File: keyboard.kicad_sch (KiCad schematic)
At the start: 295 parts

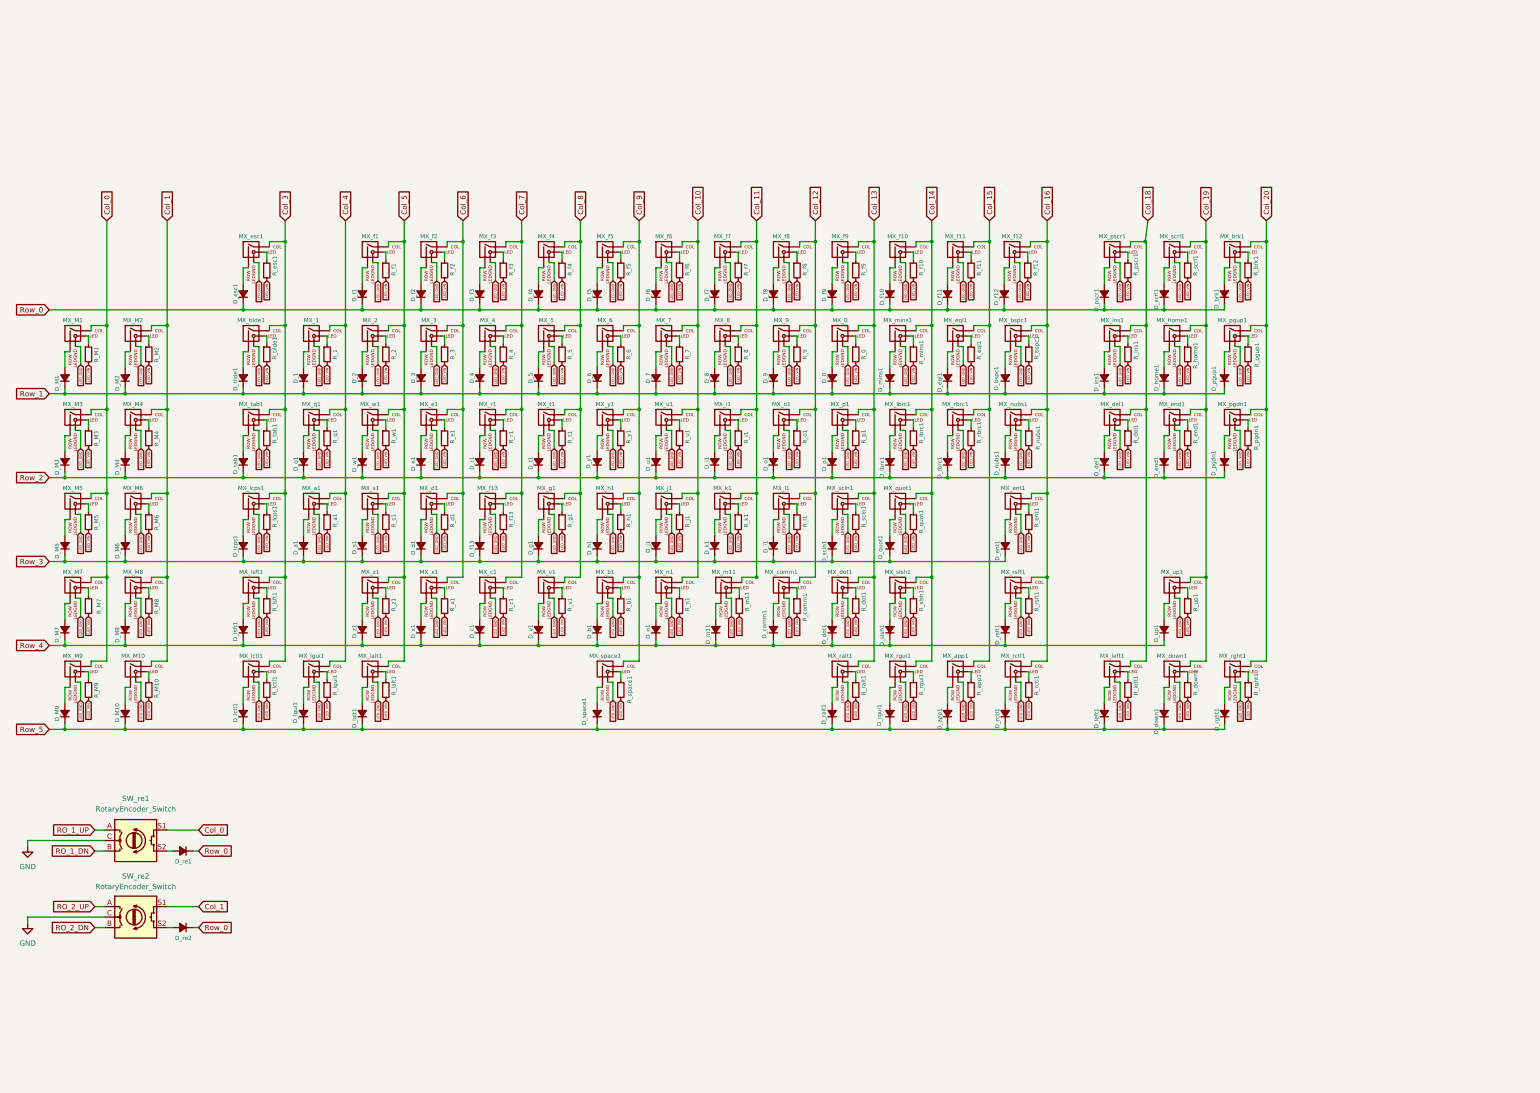
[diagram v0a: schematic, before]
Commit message: Update to plan
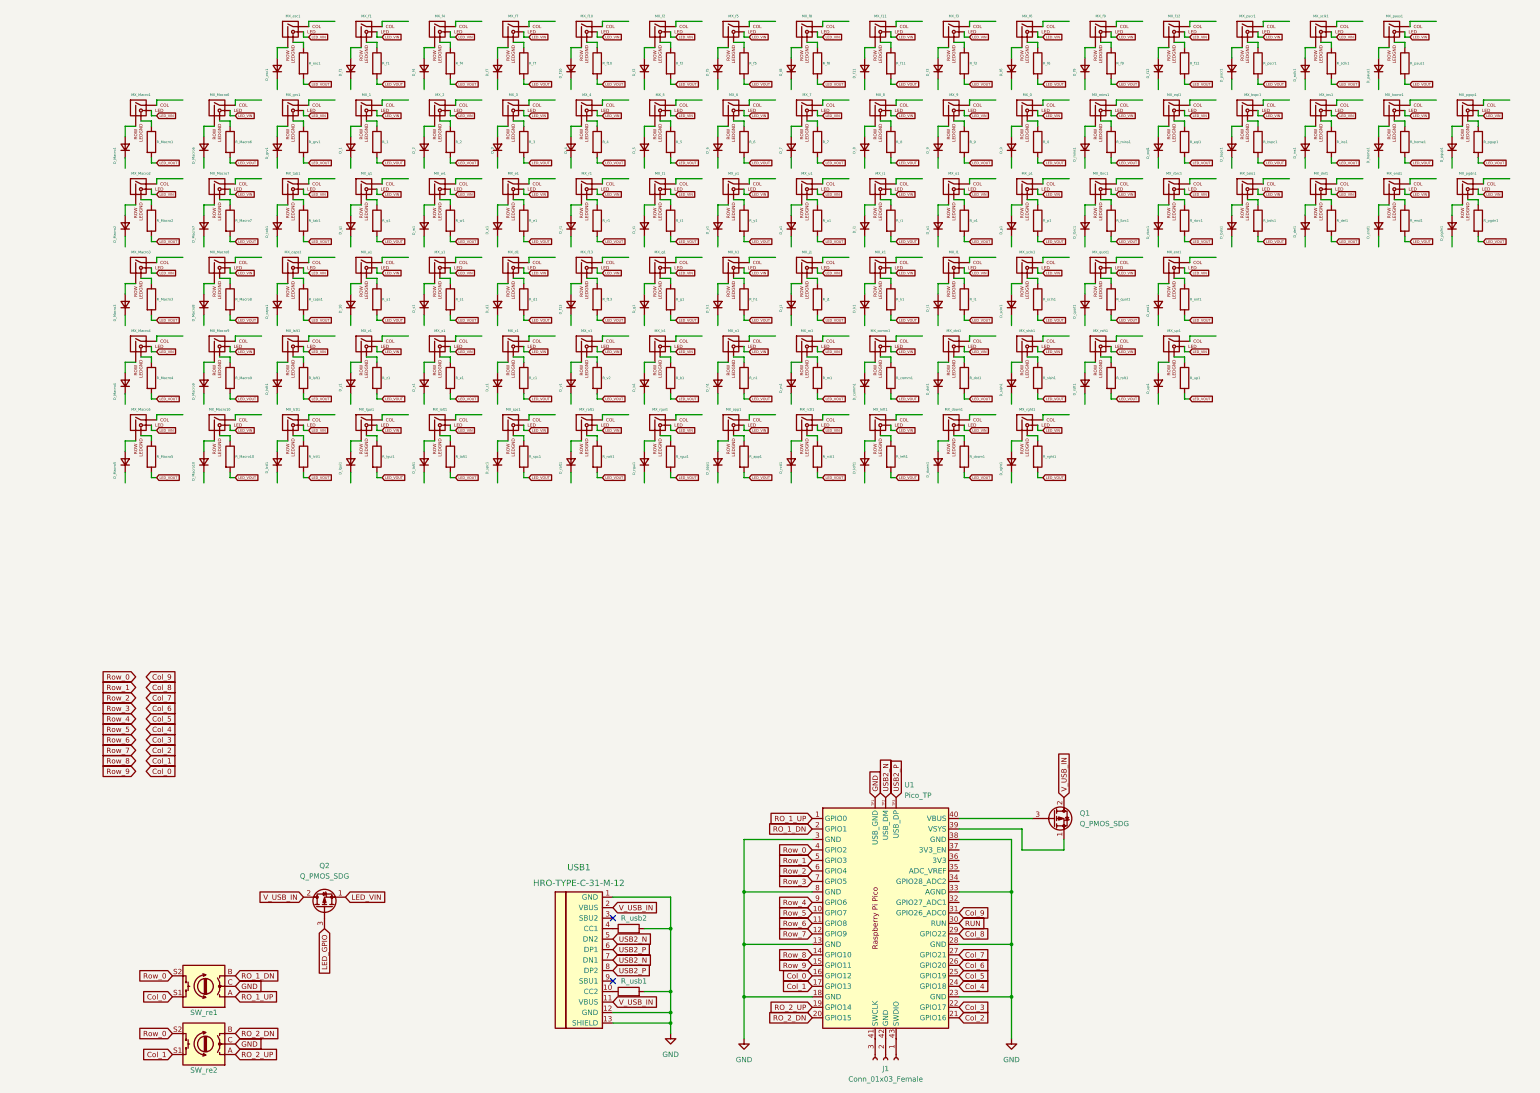
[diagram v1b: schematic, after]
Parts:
- removed D_0, D_1, D_2, D_3, D_4, D_5, D_6, D_7, D_8, D_9, D_M1, D_M10, D_M2, D_M3, D_M4, D_M5, D_M6, D_M7, D_M8, D_M9, D_a1, D_app1, D_b1, D_brk1, D_bspc1, D_c1, D_comm1, D_d1, D_del1, D_dot1, D_down1, D_e1, D_end1, D_ent1, D_eql1, D_esc1, D_f1, D_f10, D_f11, D_f12, D_f13, D_f2, D_f3, D_f4, D_f5, D_f6, D_f7, D_f8, D_f9, D_g1, D_h1, D_home1, D_i1, D_ins1, D_j1, D_k1, D_l1, D_lalt1, D_lbrc1, D_lcps1, D_lctl1, D_left1, D_lgui1, D_lsft1, D_m11, D_mins1, D_n1, D_nubs1, D_o1, D_p1, D_pgdn1, D_pgup1, D_pscr1, D_q1, D_quot1, D_r1, D_ralt1, D_rbrc1, D_rctl1, D_re1, D_re2, D_rght1, D_rgui1, D_rsft1, D_s1, D_scln1, D_scrl1, D_slsh1, D_space1, D_t1, D_tab1, D_tilde1, D_u1, D_up1, D_v1, D_w1, D_x1, D_y1, D_z1: D_Small_Filled, Diode_SMD:D_0805_2012Metric_Pad1.15x1.40mm_HandSolder, symbol Device:D_Small_Filled
- removed MX_M1, MX_M10, MX_M2, MX_M3, MX_M4, MX_M5, MX_M6, MX_M7, MX_M8, MX_M9, MX_brk1, MX_m11, MX_scrl1, MX_tilde1: MX-LED, 0_MX_Only:MXOnly-1U, symbol MX_Alps_Hybrid:MX-LED
- removed MX_lcps1: MX-LED, 0_MX_Only:MXOnly-1.75U, symbol MX_Alps_Hybrid:MX-LED
- removed MX_nubs1: MX-LED, 0_MX_Only:MXOnly-1.5U, symbol MX_Alps_Hybrid:MX-LED
- removed MX_space1: MX-LED, 0_MX_Only:MXOnly-6.25U-ReversedStabilizers, symbol MX_Alps_Hybrid:MX-LED
- removed R_0, R_1, R_2, R_3, R_4, R_5, R_6, R_7, R_8, R_9, R_M1, R_M10, R_M2, R_M3, R_M4, R_M5, R_M6, R_M7, R_M8, R_M9, R_a1, R_app1, R_b1, R_brk1, R_bspc1, R_c1, R_comm1, R_d1, R_del1, R_dot1, R_down1, R_e1, R_end1, R_ent1, R_eql1, R_esc1, R_f1, R_f10, R_f11, R_f12, R_f13, R_f2, R_f3, R_f4, R_f5, R_f6, R_f7, R_f8, R_f9, R_g1, R_h1, R_home1, R_i1, R_ins1, R_j1, R_k1, R_l1, R_lalt1, R_lbrc1, R_lcps1, R_lctl1, R_left1, R_lgui1, R_lsft1, R_m11, R_mins1, R_n1, R_nubs1, R_o1, R_p1, R_pgdn1, R_pgup1, R_pscr1, R_q1, R_quot1, R_r1, R_ralt1, R_rbrc1, R_rctl1, R_rght1, R_rgui1, R_rsft1, R_s1, R_scln1, R_scrl1, R_slsh1, R_space1, R_t1, R_tab1, R_tilde1, R_u1, R_up1, R_v1, R_w1, R_x1, R_y1, R_z1: R_Small, Resistor_SMD:R_0805_2012Metric_Pad1.20x1.40mm_HandSolder, symbol Device:R_Small
- added D_0, D_1, D_10, D_2, D_3, D_4, D_5, D_6, D_7, D_8, D_9, D_Macro1, D_Macro10, D_Macro2, D_Macro3, D_Macro4, D_Macro5, D_Macro6, D_Macro7, D_Macro8, D_Macro9, D_app1, D_b1, D_bsls1, D_bspc1, D_c1, D_caps1, D_comm1, D_d1, D_del1, D_dot1, D_down1, D_e1, D_end1, D_ent1, D_eql1, D_esc1, D_f1, D_f10, D_f11, D_f12, D_f13, D_f2, D_f3, D_f4, D_f5, D_f6, D_f7, D_f8, D_f9, D_g1, D_grv1, D_h1, D_home1, D_i1, D_ins1, D_j1, D_k1, D_l1, D_lalt1, D_lbrc1, D_lctl1, D_left1, D_lgui1, D_lsft1, D_m1, D_mins1, D_n1, D_o1, D_p1, D_paus1, D_pgdn1, D_pgup1, D_pscr1, D_q1, D_quot1, D_r1, D_ralt1, D_rbrc1, D_rctl1, D_rght1, D_rgui1, D_rsft1, D_s1, D_sclk1, D_scln1, D_slsh1, D_spc1, D_t1, D_tab1, D_u1, D_up1, D_v1, D_w1, D_x1, D_y1, D_z1: D_Small, symbol Device:D_Small
- added J1: Conn_01x03_Female, symbol Connector:Conn_01x03_Female
- added MX_Macro1, MX_Macro10, MX_Macro2, MX_Macro3, MX_Macro4, MX_Macro5, MX_Macro6, MX_Macro7, MX_Macro8, MX_Macro9, MX_grv1, MX_m1, MX_paus1, MX_sclk1: MX-LED, 0_MX_Only:MXOnly-1U, symbol MX_Alps_Hybrid:MX-LED
- added MX_bsls1: MX-LED, 0_MX_Only:MXOnly-1.5U, symbol MX_Alps_Hybrid:MX-LED
- added MX_caps1: MX-LED, 0_MX_Only:MXOnly-1.75U, symbol MX_Alps_Hybrid:MX-LED
- added MX_spc1: MX-LED, 0_MX_Only:MXOnly-6.25U-ReversedStabilizers, symbol MX_Alps_Hybrid:MX-LED
- added Q1, Q2: Q_PMOS_SDG, symbol Device:Q_PMOS_SDG
- added R_0, R_1, R_2, R_3, R_4, R_5, R_6, R_7, R_8, R_9, R_Macro1, R_Macro10, R_Macro2, R_Macro3, R_Macro4, R_Macro5, R_Macro6, R_Macro7, R_Macro8, R_Macro9, R_a1, R_app1, R_b1, R_bsls1, R_bspc1, R_c1, R_caps1, R_comm1, R_d1, R_del1, R_dot1, R_down1, R_e1, R_end1, R_ent1, R_eql1, R_esc1, R_f1, R_f10, R_f11, R_f12, R_f13, R_f2, R_f3, R_f4, R_f5, R_f6, R_f7, R_f8, R_f9, R_g1, R_grv1, R_h1, R_home1, R_i1, R_ins1, R_j1, R_k1, R_l1, R_lalt1, R_lbrc1, R_lctl1, R_left1, R_lgui1, R_lsft1, R_m1, R_mins1, R_n1, R_o1, R_p1, R_paus1, R_pgdn1, R_pgup1, R_pscr1, R_q1, R_quot1, R_r1, R_ralt1, R_rbrc1, R_rctl1, R_rght1, R_rgui1, R_rsft1, R_s1, R_sclk1, R_scln1, R_slsh1, R_spc1, R_t1, R_tab1, R_u1, R_up1, R_usb1, R_v2, R_w1, R_x1, R_y1, R_z1: R, symbol Device:R
- added R_usb2: 1, symbol Device:R
- added U1: Pico_TP, 0_MCU_RaspberryPi_and_Boards:RPi_Pico_SMD_TP, symbol 00_MCU_RaspberryPi_and_Boards:Pico_TP
- added USB1: HRO-TYPE-C-31-M-12, 0_Keebio:HRO-TYPE-C-31-M-12-Assembly, symbol 00_keebio:HRO-TYPE-C-31-M-12
- MX_bspc1: footprint 0_MX_Only:MXOnly-2U-ReversedStabilizers -> 0_MX_Only:MXOnly-2U
- MX_rgui1: footprint 0_MX_Only:MXOnly-1U -> 0_MX_Only:MXOnly-1.25U
- SW_re1, SW_re2: footprint keebio:RotaryEncoder_Alps_EC11E-Switch_Vertical_H20mm -> 0_Keebio:RotaryEncoder_EC11
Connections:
- net Col_0: now also U1.16 (GPIO12)
- net Col_1: now also U1.17 (GPIO13)
- net Col_3: now also U1.22 (GPIO17); no longer MX_esc1.1 (COL), MX_lctl1.1 (COL), MX_lsft1.1 (COL), MX_tab1.1 (COL)
- net Col_4: now also U1.24 (GPIO18); no longer MX_1.1 (COL), MX_a1.1 (COL), MX_lgui1.1 (COL), MX_q1.1 (COL)
- net Col_5: now also U1.25 (GPIO19); no longer MX_2.1 (COL), MX_f1.1 (COL), MX_lalt1.1 (COL), MX_s1.1 (COL), MX_w1.1 (COL), MX_z1.1 (COL)
- net Col_6: now also U1.26 (GPIO20); no longer MX_3.1 (COL), MX_d1.1 (COL), MX_e1.1 (COL), MX_f2.1 (COL), MX_x1.1 (COL)
- net Col_7: now also U1.27 (GPIO21); no longer MX_4.1 (COL), MX_c1.1 (COL), MX_f13.1 (COL), MX_f3.1 (COL), MX_r1.1 (COL)
- net Col_8: now also U1.29 (GPIO22); no longer MX_5.1 (COL), MX_f4.1 (COL), MX_g1.1 (COL), MX_t1.1 (COL), MX_v1.1 (COL)
- net Col_9: now also U1.31 (GPIO26_ADC0); no longer MX_6.1 (COL), MX_b1.1 (COL), MX_f5.1 (COL), MX_h1.1 (COL), MX_y1.1 (COL)
- net GND: now also R_usb1.2, R_usb2.2, U1.13 (GND), U1.18 (GND), U1.23 (GND), U1.28 (GND), U1.3 (GND), U1.33 (AGND), U1.38 (GND), U1.8 (GND), U1.TP1 (USB_GND), USB1.1 (GND), USB1.12 (GND), USB1.13 (SHIELD)
- net LED_VIN: now also MX_0.3 (LED), MX_1.3 (LED), MX_2.3 (LED), MX_3.3 (LED), MX_4.3 (LED), MX_5.3 (LED), MX_6.3 (LED), MX_7.3 (LED), MX_8.3 (LED), MX_9.3 (LED), MX_a1.3 (LED), MX_app1.3 (LED), MX_b1.3 (LED), MX_bspc1.3 (LED), MX_c1.3 (LED), MX_comm1.3 (LED), MX_d1.3 (LED), MX_del1.3 (LED), MX_dot1.3 (LED), MX_down1.3 (LED), MX_e1.3 (LED), MX_end1.3 (LED), MX_ent1.3 (LED), MX_eql1.3 (LED), MX_esc1.3 (LED), MX_f1.3 (LED), MX_f10.3 (LED), MX_f11.3 (LED), MX_f12.3 (LED), MX_f13.3 (LED), MX_f2.3 (LED), MX_f3.3 (LED), MX_f4.3 (LED), MX_f5.3 (LED), MX_f6.3 (LED), MX_f7.3 (LED), MX_f8.3 (LED), MX_f9.3 (LED), MX_g1.3 (LED), MX_h1.3 (LED), MX_home1.3 (LED), MX_i1.3 (LED), MX_ins1.3 (LED), MX_j1.3 (LED), MX_k1.3 (LED), MX_l1.3 (LED), MX_lalt1.3 (LED), MX_lbrc1.3 (LED), MX_lctl1.3 (LED), MX_left1.3 (LED), MX_lgui1.3 (LED), MX_lsft1.3 (LED), MX_mins1.3 (LED), MX_n1.3 (LED), MX_o1.3 (LED), MX_p1.3 (LED), MX_pgdn1.3 (LED), MX_pgup1.3 (LED), MX_pscr1.3 (LED), MX_q1.3 (LED), MX_quot1.3 (LED), MX_r1.3 (LED), MX_ralt1.3 (LED), MX_rbrc1.3 (LED), MX_rctl1.3 (LED), MX_rght1.3 (LED), MX_rgui1.3 (LED), MX_rsft1.3 (LED), MX_s1.3 (LED), MX_scln1.3 (LED), MX_slsh1.3 (LED), MX_t1.3 (LED), MX_tab1.3 (LED), MX_u1.3 (LED), MX_up1.3 (LED), MX_v1.3 (LED), MX_w1.3 (LED), MX_x1.3 (LED), MX_y1.3 (LED), MX_z1.3 (LED), MX_Macro1.3 (LED), MX_Macro10.3 (LED), MX_Macro2.3 (LED), MX_Macro3.3 (LED), MX_Macro4.3 (LED), MX_Macro5.3 (LED), MX_Macro6.3 (LED), MX_Macro7.3 (LED), MX_Macro8.3 (LED), MX_Macro9.3 (LED), MX_bsls1.3 (LED), MX_caps1.3 (LED), MX_grv1.3 (LED), MX_m1.3 (LED), MX_paus1.3 (LED), MX_sclk1.3 (LED), MX_spc1.3 (LED), Q2.1 (S)
- net RO_1_UP: now also U1.1 (GPIO0)
- net RO_2_DN: now also U1.20 (GPIO15)
- net RO_2_UP: now also U1.19 (GPIO14)
- net Row_0: now also SW_re1.S2, SW_re2.S2, U1.4 (GPIO2)
- net Row_1: now also U1.5 (GPIO3)
- net Row_2: now also U1.6 (GPIO4)
- net Row_3: now also U1.7 (GPIO5)
- net Row_4: now also U1.9 (GPIO6)
- net Row_5: now also U1.10 (GPIO7)
- net at MX_pscr1.2 (ROW): now also D_pscr1.2 (A)
- net at MX_p1.2 (ROW): now also D_p1.2 (A)
- net at MX_end1.2 (ROW): now also D_end1.2 (A)
- net at MX_ralt1.2 (ROW): now also D_ralt1.2 (A)
- net at MX_o1.2 (ROW): now also D_o1.2 (A)
- net at MX_4.2 (ROW): now also D_4.2 (A)
- net at MX_y1.2 (ROW): now also D_y1.2 (A)
- net at MX_l1.2 (ROW): now also D_l1.2 (A)
- net at MX_6.2 (ROW): now also D_6.2 (A)
- net at MX_pgup1.2 (ROW): now also D_pgup1.2 (A)
- net at MX_eql1.2 (ROW): now also D_eql1.2 (A)
- net at MX_n1.2 (ROW): now also D_n1.2 (A)
- net at MX_j1.2 (ROW): now also D_j1.2 (A)
- net at MX_f5.2 (ROW): now also D_f5.2 (A)
- net at MX_f3.2 (ROW): now also D_f3.2 (A)
- net at MX_f7.2 (ROW): now also D_f7.2 (A)
- net at MX_rght1.2 (ROW): now also D_rght1.2 (A)
- net at MX_u1.2 (ROW): now also D_u1.2 (A)
- net at MX_rbrc1.2 (ROW): now also D_rbrc1.2 (A)
- net at MX_7.2 (ROW): now also D_7.2 (A)
- net at MX_pgdn1.2 (ROW): now also D_pgdn1.2 (A)
- net at MX_mins1.2 (ROW): now also D_mins1.2 (A)
- net at MX_x1.2 (ROW): now also D_x1.2 (A)
- net at MX_f4.2 (ROW): now also D_f4.2 (A)
- net at MX_f9.2 (ROW): now also D_f9.2 (A)
- net at MX_b1.2 (ROW): now also D_b1.2 (A)
- net at MX_dot1.2 (ROW): now also D_dot1.2 (A)
- net at MX_left1.2 (ROW): now also D_left1.2 (A)
- net at MX_f12.2 (ROW): now also D_f12.2 (A)
- net at MX_lalt1.2 (ROW): now also D_lalt1.2 (A)
- net at MX_r1.2 (ROW): now also D_r1.2 (A)
- net at MX_3.2 (ROW): now also D_3.2 (A)
- net at MX_g1.2 (ROW): now also D_g1.2 (A)
- net at MX_ent1.2 (ROW): now also D_ent1.2 (A)
- net at MX_1.2 (ROW): now also D_1.2 (A)
- net at MX_k1.2 (ROW): now also D_k1.2 (A)
- net at MX_f8.2 (ROW): now also D_f8.2 (A)
- net at MX_ins1.2 (ROW): now also D_ins1.2 (A)
- net at MX_c1.2 (ROW): now also D_c1.2 (A)
- net at MX_rsft1.2 (ROW): now also D_rsft1.2 (A)
- net at MX_f10.2 (ROW): now also D_f10.2 (A)
- net at MX_z1.2 (ROW): now also D_z1.2 (A)
- net at MX_e1.2 (ROW): now also D_e1.2 (A)
- net at MX_f1.2 (ROW): now also D_f1.2 (A)
- net at MX_d1.2 (ROW): now also D_d1.2 (A)
- net at MX_t1.2 (ROW): now also D_t1.2 (A)
- net at MX_9.2 (ROW): now also D_9.2 (A)
- net at MX_w1.2 (ROW): now also D_w1.2 (A)
- net at MX_0.2 (ROW): now also D_0.2 (A)
- net at MX_rgui1.2 (ROW): now also D_rgui1.2 (A)
- net at MX_home1.2 (ROW): now also D_home1.2 (A)
- net at MX_bspc1.2 (ROW): now also D_bspc1.2 (A)
- net at MX_s1.2 (ROW): now also D_s1.2 (A)
- net at MX_rctl1.2 (ROW): now also D_rctl1.2 (A)
- net at MX_8.2 (ROW): now also D_8.2 (A)
- net at MX_quot1.2 (ROW): now also D_quot1.2 (A)
- net at MX_comm1.2 (ROW): now also D_comm1.2 (A)
- net at MX_f11.2 (ROW): now also D_f11.2 (A)
- net at MX_del1.2 (ROW): now also D_del1.2 (A)
- net at MX_lgui1.2 (ROW): now also D_lgui1.2 (A)
- net at MX_v1.2 (ROW): now also D_v1.2 (A)
- net at MX_h1.2 (ROW): now also D_h1.2 (A)
- net at MX_slsh1.2 (ROW): now also D_slsh1.2 (A)
- net at MX_lsft1.2 (ROW): now also D_lsft1.2 (A)
- net at MX_lbrc1.2 (ROW): now also D_lbrc1.2 (A)
- net at MX_tab1.2 (ROW): now also D_tab1.2 (A)
- net at MX_f13.2 (ROW): now also D_f13.2 (A)
- net at MX_f6.2 (ROW): now also D_f6.2 (A)
- net at MX_5.2 (ROW): now also D_5.2 (A)
- net at MX_scln1.2 (ROW): now also D_scln1.2 (A)
- net at MX_app1.2 (ROW): now also D_app1.2 (A)
- net at MX_a1.2 (ROW): now also D_10.2 (A)
- net at MX_down1.2 (ROW): now also D_down1.2 (A)
- net at MX_q1.2 (ROW): now also D_q1.2 (A)
- net at MX_f2.2 (ROW): now also D_f2.2 (A)
- net at MX_esc1.2 (ROW): now also D_esc1.2 (A)
- net at MX_lctl1.2 (ROW): now also D_lctl1.2 (A)
- net at MX_i1.2 (ROW): now also D_i1.2 (A)
- net at MX_up1.2 (ROW): now also D_up1.2 (A)
- net at MX_2.2 (ROW): now also D_2.2 (A)
- removed net Col_10: MX_7.1 (COL), MX_f6.1 (COL), MX_j1.1 (COL), MX_n1.1 (COL), MX_u1.1 (COL)
- removed net Col_11: MX_8.1 (COL), MX_f7.1 (COL), MX_i1.1 (COL), MX_k1.1 (COL)
- removed net Col_12: MX_9.1 (COL), MX_comm1.1 (COL), MX_f8.1 (COL), MX_l1.1 (COL), MX_o1.1 (COL)
- removed net Col_13: MX_0.1 (COL), MX_dot1.1 (COL), MX_f9.1 (COL), MX_p1.1 (COL), MX_ralt1.1 (COL), MX_scln1.1 (COL)
- removed net Col_14: MX_f10.1 (COL), MX_lbrc1.1 (COL), MX_mins1.1 (COL), MX_quot1.1 (COL), MX_rgui1.1 (COL), MX_slsh1.1 (COL)
- removed net Col_15: MX_app1.1 (COL), MX_eql1.1 (COL), MX_f11.1 (COL), MX_rbrc1.1 (COL)
- removed net Col_16: MX_bspc1.1 (COL), MX_ent1.1 (COL), MX_f12.1 (COL), MX_rctl1.1 (COL), MX_rsft1.1 (COL)
- removed net Col_18: MX_del1.1 (COL), MX_ins1.1 (COL), MX_left1.1 (COL), MX_pscr1.1 (COL)
- removed net Col_19: MX_down1.1 (COL), MX_end1.1 (COL), MX_home1.1 (COL), MX_up1.1 (COL)
- removed net Col_20: MX_pgdn1.1 (COL), MX_pgup1.1 (COL), MX_rght1.1 (COL)
- removed net LED_GND: MX_0.4 (LEDGND), MX_1.4 (LEDGND), MX_2.4 (LEDGND), MX_3.4 (LEDGND), MX_4.4 (LEDGND), MX_5.4 (LEDGND), MX_6.4 (LEDGND), MX_7.4 (LEDGND), MX_8.4 (LEDGND), MX_9.4 (LEDGND), MX_a1.4 (LEDGND), MX_app1.4 (LEDGND), MX_b1.4 (LEDGND), MX_bspc1.4 (LEDGND), MX_c1.4 (LEDGND), MX_comm1.4 (LEDGND), MX_d1.4 (LEDGND), MX_del1.4 (LEDGND), MX_dot1.4 (LEDGND), MX_down1.4 (LEDGND), MX_e1.4 (LEDGND), MX_end1.4 (LEDGND), MX_ent1.4 (LEDGND), MX_eql1.4 (LEDGND), MX_esc1.4 (LEDGND), MX_f1.4 (LEDGND), MX_f10.4 (LEDGND), MX_f11.4 (LEDGND), MX_f12.4 (LEDGND), MX_f13.4 (LEDGND), MX_f2.4 (LEDGND), MX_f3.4 (LEDGND), MX_f4.4 (LEDGND), MX_f5.4 (LEDGND), MX_f6.4 (LEDGND), MX_f7.4 (LEDGND), MX_f8.4 (LEDGND), MX_f9.4 (LEDGND), MX_g1.4 (LEDGND), MX_h1.4 (LEDGND), MX_home1.4 (LEDGND), MX_i1.4 (LEDGND), MX_ins1.4 (LEDGND), MX_j1.4 (LEDGND), MX_k1.4 (LEDGND), MX_l1.4 (LEDGND), MX_lalt1.4 (LEDGND), MX_lbrc1.4 (LEDGND), MX_lctl1.4 (LEDGND), MX_left1.4 (LEDGND), MX_lgui1.4 (LEDGND), MX_lsft1.4 (LEDGND), MX_mins1.4 (LEDGND), MX_n1.4 (LEDGND), MX_o1.4 (LEDGND), MX_p1.4 (LEDGND), MX_pgdn1.4 (LEDGND), MX_pgup1.4 (LEDGND), MX_pscr1.4 (LEDGND), MX_q1.4 (LEDGND), MX_quot1.4 (LEDGND), MX_r1.4 (LEDGND), MX_ralt1.4 (LEDGND), MX_rbrc1.4 (LEDGND), MX_rctl1.4 (LEDGND), MX_rght1.4 (LEDGND), MX_rgui1.4 (LEDGND), MX_rsft1.4 (LEDGND), MX_s1.4 (LEDGND), MX_scln1.4 (LEDGND), MX_slsh1.4 (LEDGND), MX_t1.4 (LEDGND), MX_tab1.4 (LEDGND), MX_u1.4 (LEDGND), MX_up1.4 (LEDGND), MX_v1.4 (LEDGND), MX_w1.4 (LEDGND), MX_x1.4 (LEDGND), MX_y1.4 (LEDGND), MX_z1.4 (LEDGND)
- new net: MX_f7.4 (LEDGND), R_f7.1
- new net: D_m1.2 (A), MX_m1.2 (ROW)
- new net: MX_ralt1.4 (LEDGND), R_ralt1.1
- new net: MX_pscr1.4 (LEDGND), R_pscr1.1
- new net: J1.1 (Pin_1), U1.43 (SWDIO)
- new net: J1.2 (Pin_2), U1.42 (GND)
- new net: J1.3 (Pin_3), U1.41 (SWCLK)
- new net: MX_pgdn1.4 (LEDGND), R_pgdn1.1
- new net: MX_p1.4 (LEDGND), R_p1.1
- new net: MX_f1.4 (LEDGND), R_f1.1
- new net: MX_3.4 (LEDGND), R_3.1
- new net: D_caps1.2 (A), MX_caps1.2 (ROW)
- new net: MX_caps1.4 (LEDGND), R_caps1.1
- new net: MX_y1.4 (LEDGND), R_y1.1
- new net: MX_r1.4 (LEDGND), R_r1.1
- new net: MX_ins1.4 (LEDGND), R_ins1.1
- new net: MX_Macro1.4 (LEDGND), R_Macro1.1
- new net: MX_f2.4 (LEDGND), R_f2.1
- new net: MX_f10.4 (LEDGND), R_f10.1
- new net: MX_quot1.4 (LEDGND), R_quot1.1
- new net: MX_esc1.4 (LEDGND), R_esc1.1
- new net: MX_q1.4 (LEDGND), R_q1.1
- new net: MX_lalt1.4 (LEDGND), R_lalt1.1
- new net: D_bsls1.2 (A), MX_bsls1.2 (ROW)
- new net: MX_bsls1.4 (LEDGND), R_bsls1.1
- new net: MX_dot1.4 (LEDGND), R_dot1.1
- new net: MX_5.4 (LEDGND), R_5.1
- new net: MX_down1.4 (LEDGND), R_down1.1
- new net: MX_tab1.4 (LEDGND), R_tab1.1
- new net: R_usb1.1, USB1.10 (CC2)
- new net: R_usb2.1, USB1.4 (CC1)
- new net: MX_scln1.4 (LEDGND), R_scln1.1
- new net: MX_f13.4 (LEDGND), R_f13.1
- new net: MX_d1.4 (LEDGND), R_d1.1
- new net: MX_x1.4 (LEDGND), R_x1.1
- new net: D_Macro9.2 (A), MX_Macro9.2 (ROW)
- new net: MX_rgui1.4 (LEDGND), R_rgui1.1
- new net: MX_e1.4 (LEDGND), R_e1.1
- new net: MX_f5.4 (LEDGND), R_f5.1
- new net: D_spc1.2 (A), MX_spc1.2 (ROW)
- new net: MX_spc1.4 (LEDGND), R_spc1.1
- new net: D_Macro1.2 (A), MX_Macro1.2 (ROW)
- new net: MX_f6.4 (LEDGND), R_f6.1
- new net: MX_b1.4 (LEDGND), R_b1.1
- new net: D_Macro8.2 (A), MX_Macro8.2 (ROW)
- new net: MX_Macro8.4 (LEDGND), R_Macro8.1
- new net: MX_l1.4 (LEDGND), R_l1.1
- new net: MX_t1.4 (LEDGND), R_t1.1
- new net: MX_Macro10.4 (LEDGND), R_Macro10.1
- new net: MX_eql1.4 (LEDGND), R_eql1.1
- new net: MX_rbrc1.4 (LEDGND), R_rbrc1.1
- new net: MX_v1.4 (LEDGND), R_v2.1
- new net: MX_lbrc1.4 (LEDGND), R_lbrc1.1
- new net: MX_4.4 (LEDGND), R_4.1
- new net: MX_8.4 (LEDGND), R_8.1
- new net: MX_a1.4 (LEDGND), R_a1.1
- new net: MX_f9.4 (LEDGND), R_f9.1
- new net: MX_rsft1.4 (LEDGND), R_rsft1.1
- new net: MX_home1.4 (LEDGND), R_home1.1
- new net: MX_h1.4 (LEDGND), R_h1.1
- new net: MX_f4.4 (LEDGND), R_f4.1
- new net: MX_k1.4 (LEDGND), R_k1.1
- new net: MX_rctl1.4 (LEDGND), R_rctl1.1
- new net: MX_1.4 (LEDGND), R_1.1
- new net: MX_up1.4 (LEDGND), R_up1.1
- new net: MX_m1.4 (LEDGND), R_m1.1
- new net: D_Macro6.2 (A), MX_Macro6.2 (ROW)
- new net: MX_comm1.4 (LEDGND), R_comm1.1
- new net: Q1.1 (S), U1.39 (VSYS)
- new net: Q1.3 (G), U1.40 (VBUS)
- new net: MX_s1.4 (LEDGND), R_s1.1
- new net: MX_7.4 (LEDGND), R_7.1
- new net: MX_o1.4 (LEDGND), R_o1.1
- new net: MX_Macro9.4 (LEDGND), R_Macro9.1
- new net: MX_del1.4 (LEDGND), R_del1.1
- new net: MX_pgup1.4 (LEDGND), R_pgup1.1
- new net: MX_z1.4 (LEDGND), R_z1.1
- new net: MX_left1.4 (LEDGND), R_left1.1
- new net: MX_slsh1.4 (LEDGND), R_slsh1.1
- new net: MX_u1.4 (LEDGND), R_u1.1
- new net: D_sclk1.2 (A), MX_sclk1.2 (ROW)
- new net: MX_rght1.4 (LEDGND), R_rght1.1
- new net: MX_2.4 (LEDGND), R_2.1
- new net: MX_mins1.4 (LEDGND), R_mins1.1
- new net: D_paus1.2 (A), MX_paus1.2 (ROW)
- new net: MX_g1.4 (LEDGND), R_g1.1
- new net: D_grv1.2 (A), MX_grv1.2 (ROW)
- new net: D_Macro10.2 (A), MX_Macro10.2 (ROW)
- new net: MX_grv1.4 (LEDGND), R_grv1.1
- new net: MX_Macro5.4 (LEDGND), R_Macro5.1
- new net: MX_6.4 (LEDGND), R_6.1
- new net: MX_lgui1.4 (LEDGND), R_lgui1.1
- new net: D_Macro7.2 (A), MX_Macro7.2 (ROW)
- new net: MX_Macro7.4 (LEDGND), R_Macro7.1
- new net: MX_lctl1.4 (LEDGND), R_lctl1.1
- new net: MX_Macro2.4 (LEDGND), R_Macro2.1
- new net: MX_f8.4 (LEDGND), R_f8.1
- new net: D_Macro3.2 (A), MX_Macro3.2 (ROW)
- new net: MX_Macro3.4 (LEDGND), R_Macro3.1
- new net: MX_bspc1.4 (LEDGND), R_bspc1.1
- new net: MX_0.4 (LEDGND), R_0.1
- new net: MX_i1.4 (LEDGND), R_i1.1
- new net: D_Macro4.2 (A), MX_Macro4.2 (ROW)
- new net: MX_lsft1.4 (LEDGND), R_lsft1.1
- new net: MX_9.4 (LEDGND), R_9.1
- new net: MX_f11.4 (LEDGND), R_f11.1
- new net: MX_w1.4 (LEDGND), R_w1.1
- new net: MX_c1.4 (LEDGND), R_c1.1
- new net: MX_j1.4 (LEDGND), R_j1.1
- new net: MX_ent1.4 (LEDGND), R_ent1.1
- new net: MX_end1.4 (LEDGND), R_end1.1
- new net: MX_Macro4.4 (LEDGND), R_Macro4.1
- new net: MX_sclk1.4 (LEDGND), R_sclk1.1
- new net: D_Macro2.2 (A), MX_Macro2.2 (ROW)
- new net: MX_n1.4 (LEDGND), R_n1.1
- new net: MX_app1.4 (LEDGND), R_app1.1
- new net: MX_paus1.4 (LEDGND), R_paus1.1
- new net: MX_Macro6.4 (LEDGND), R_Macro6.1
- new net: MX_f3.4 (LEDGND), R_f3.1
- new net: MX_f12.4 (LEDGND), R_f12.1
- new net: D_Macro5.2 (A), MX_Macro5.2 (ROW)
- new net Col_2: U1.21 (GPIO16)
- new net LED_GPIO: Q2.3 (G)
- new net LED_VOUT: R_0.2, R_1.2, R_2.2, R_3.2, R_4.2, R_5.2, R_6.2, R_7.2, R_8.2, R_9.2, R_Macro1.2, R_Macro10.2, R_Macro2.2, R_Macro3.2, R_Macro4.2, R_Macro5.2, R_Macro6.2, R_Macro7.2, R_Macro8.2, R_Macro9.2, R_a1.2, R_app1.2, R_b1.2, R_bsls1.2, R_bspc1.2, R_c1.2, R_caps1.2, R_comm1.2, R_d1.2, R_del1.2, R_dot1.2, R_down1.2, R_e1.2, R_end1.2, R_ent1.2, R_eql1.2, R_esc1.2, R_f1.2, R_f10.2, R_f11.2, R_f12.2, R_f13.2, R_f2.2, R_f3.2, R_f4.2, R_f5.2, R_f6.2, R_f7.2, R_f8.2, R_f9.2, R_g1.2, R_grv1.2, R_h1.2, R_home1.2, R_i1.2, R_ins1.2, R_j1.2, R_k1.2, R_l1.2, R_lalt1.2, R_lbrc1.2, R_lctl1.2, R_left1.2, R_lgui1.2, R_lsft1.2, R_m1.2, R_mins1.2, R_n1.2, R_o1.2, R_p1.2, R_paus1.2, R_pgdn1.2, R_pgup1.2, R_pscr1.2, R_q1.2, R_quot1.2, R_r1.2, R_ralt1.2, R_rbrc1.2, R_rctl1.2, R_rght1.2, R_rgui1.2, R_rsft1.2, R_s1.2, R_sclk1.2, R_scln1.2, R_slsh1.2, R_spc1.2, R_t1.2, R_tab1.2, R_u1.2, R_up1.2, R_v2.2, R_w1.2, R_x1.2, R_y1.2, R_z1.2
- new net RUN: U1.30 (RUN)
- new net Row_6: U1.11 (GPIO8)
- new net Row_7: U1.12 (GPIO9)
- new net Row_8: U1.14 (GPIO10)
- new net Row_9: U1.15 (GPIO11)
- new net USB2_N: U1.TP2 (USB_DM), USB1.5 (DN2), USB1.7 (DN1)
- new net USB2_P: U1.TP3 (USB_DP), USB1.6 (DP1), USB1.8 (DP2)
- new net V_USB_IN: Q1.2 (D), Q2.2 (D), USB1.11 (VBUS), USB1.2 (VBUS)
- no-connect marks 0 -> 2
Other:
- moved on the sheet: SW_re1, SW_re2

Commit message: Keyboard
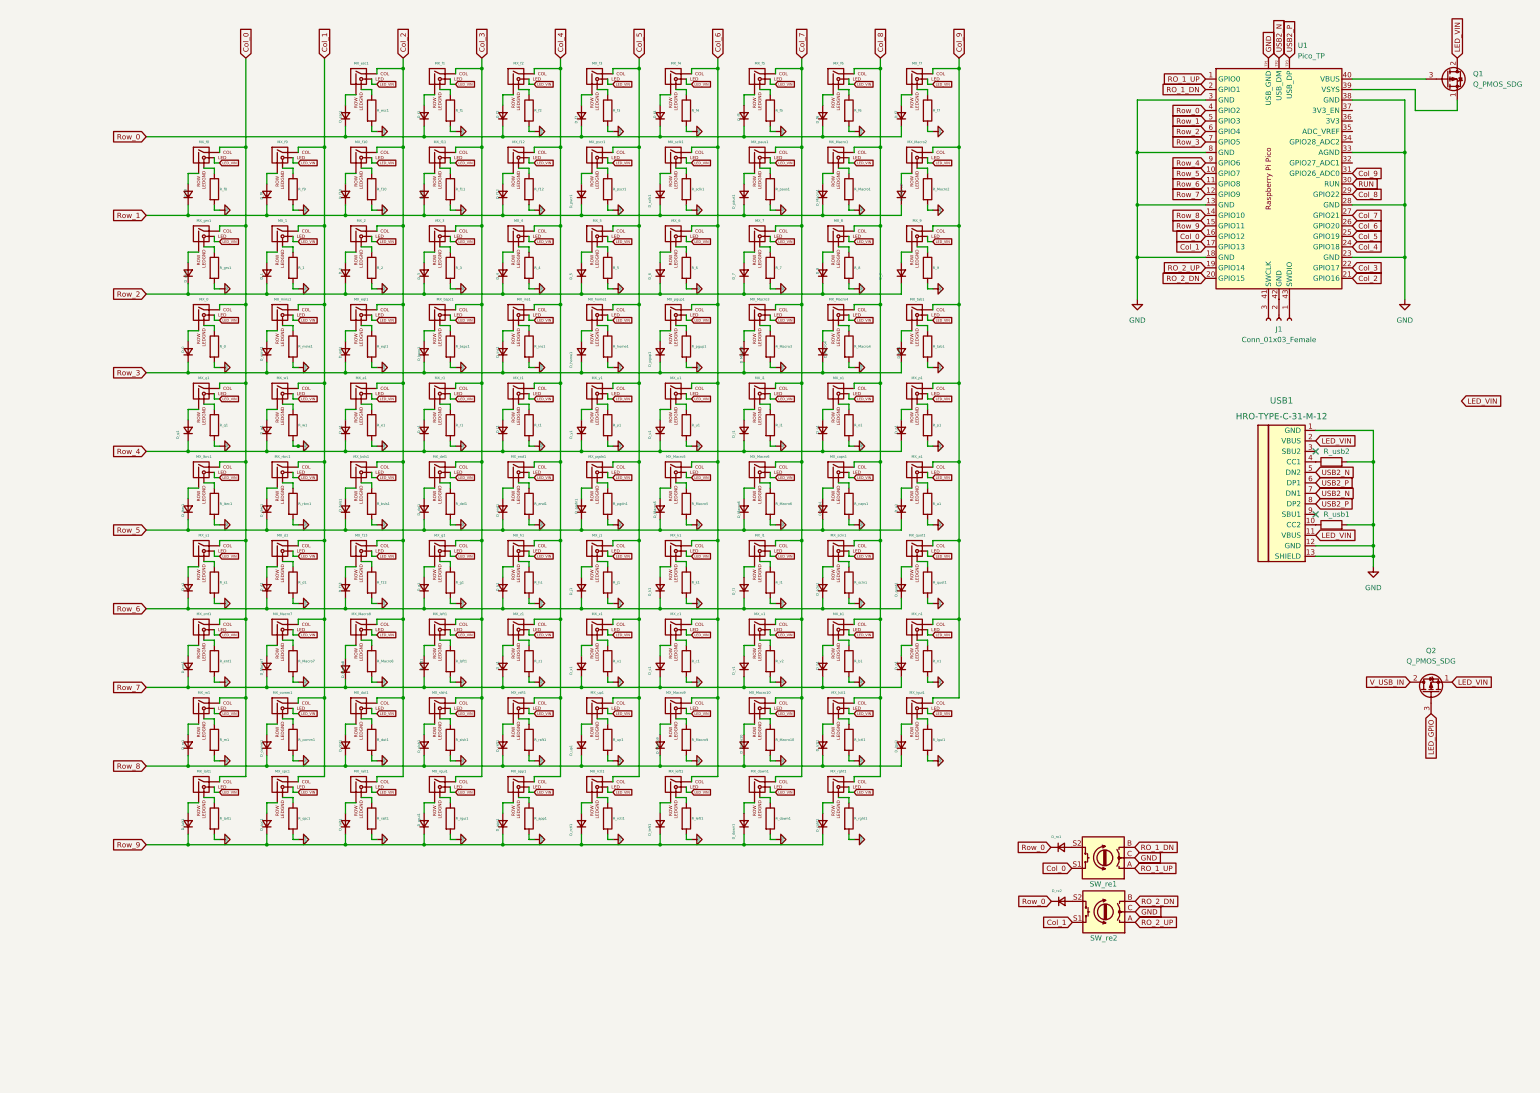
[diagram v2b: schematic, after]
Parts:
- added D_re1, D_re2: D_Small, Diode_SMD:D_0805_2012Metric_Pad1.15x1.40mm_HandSolder, symbol Device:D_Small
- D_0, D_1, D_2, D_3, D_4, D_5, D_6, D_7, D_8, D_9, D_Macro1, D_Macro10, D_Macro2, D_Macro3, D_Macro4, D_Macro5, D_Macro6, D_Macro7, D_Macro8, D_Macro9, D_app1, D_b1, D_bsls1, D_bspc1, D_c1, D_caps1, D_comm1, D_d1, D_del1, D_dot1, D_down1, D_e1, D_end1, D_ent1, D_eql1, D_esc1, D_f1, D_f10, D_f11, D_f12, D_f13, D_f2, D_f3, D_f4, D_f5, D_f6, D_f7, D_f8, D_f9, D_g1, D_grv1, D_h1, D_home1, D_i1, D_ins1, D_j1, D_k1, D_l1, D_lalt1, D_lbrc1, D_lctl1, D_left1, D_lgui1, D_lsft1, D_m1, D_mins1, D_n1, D_o1, D_p1, D_paus1, D_pgdn1, D_pgup1, D_pscr1, D_q1, D_quot1, D_r1, D_ralt1, D_rbrc1, D_rctl1, D_rght1, D_rgui1, D_rsft1, D_s1, D_sclk1, D_scln1, D_slsh1, D_spc1, D_t1, D_tab1, D_u1, D_up1, D_v1, D_w1, D_x1, D_y1, D_z1: footprint (none) -> Diode_SMD:D_0805_2012Metric_Pad1.15x1.40mm_HandSolder
- D_a1: renamed from D_10; footprint (none) -> Diode_SMD:D_0805_2012Metric_Pad1.15x1.40mm_HandSolder
- R_0, R_1, R_2, R_3, R_4, R_5, R_6, R_7, R_8, R_9, R_Macro1, R_Macro10, R_Macro2, R_Macro3, R_Macro4, R_Macro5, R_Macro6, R_Macro7, R_Macro8, R_Macro9, R_a1, R_app1, R_b1, R_bsls1, R_bspc1, R_c1, R_caps1, R_comm1, R_d1, R_del1, R_dot1, R_down1, R_e1, R_end1, R_ent1, R_eql1, R_esc1, R_f1, R_f10, R_f11, R_f12, R_f13, R_f2, R_f3, R_f4, R_f5, R_f6, R_f7, R_f8, R_f9, R_g1, R_grv1, R_h1, R_home1, R_i1, R_ins1, R_j1, R_k1, R_l1, R_lalt1, R_lbrc1, R_lctl1, R_left1, R_lgui1, R_lsft1, R_m1, R_mins1, R_n1, R_o1, R_p1, R_paus1, R_pgdn1, R_pgup1, R_pscr1, R_q1, R_quot1, R_r1, R_ralt1, R_rbrc1, R_rctl1, R_rght1, R_rgui1, R_rsft1, R_s1, R_sclk1, R_scln1, R_slsh1, R_spc1, R_t1, R_tab1, R_u1, R_up1, R_usb1, R_usb2, R_v2, R_w1, R_x1, R_y1, R_z1: footprint (none) -> Resistor_SMD:R_0805_2012Metric_Pad1.20x1.40mm_HandSolder
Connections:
- net Col_0: now also MX_0.1 (COL), MX_ent1.1 (COL), MX_f8.1 (COL), MX_grv1.1 (COL), MX_lalt1.1 (COL), MX_lbrc1.1 (COL), MX_m1.1 (COL), MX_q1.1 (COL), MX_s1.1 (COL)
- net Col_1: now also MX_1.1 (COL), MX_Macro7.1 (COL), MX_comm1.1 (COL), MX_d1.1 (COL), MX_f9.1 (COL), MX_mins1.1 (COL), MX_rbrc1.1 (COL), MX_spc1.1 (COL), MX_w1.1 (COL)
- net Col_2: now also MX_2.1 (COL), MX_Macro8.1 (COL), MX_bsls1.1 (COL), MX_dot1.1 (COL), MX_e1.1 (COL), MX_eql1.1 (COL), MX_esc1.1 (COL), MX_f10.1 (COL), MX_f13.1 (COL), MX_ralt1.1 (COL)
- net Col_3: now also MX_3.1 (COL), MX_bspc1.1 (COL), MX_del1.1 (COL), MX_f1.1 (COL), MX_f11.1 (COL), MX_g1.1 (COL), MX_lsft1.1 (COL), MX_r1.1 (COL), MX_rgui1.1 (COL), MX_slsh1.1 (COL)
- net Col_4: now also MX_4.1 (COL), MX_app1.1 (COL), MX_end1.1 (COL), MX_f12.1 (COL), MX_f2.1 (COL), MX_h1.1 (COL), MX_ins1.1 (COL), MX_rsft1.1 (COL), MX_t1.1 (COL), MX_z1.1 (COL)
- net Col_5: now also MX_5.1 (COL), MX_f3.1 (COL), MX_home1.1 (COL), MX_j1.1 (COL), MX_pgdn1.1 (COL), MX_pscr1.1 (COL), MX_rctl1.1 (COL), MX_up1.1 (COL), MX_x1.1 (COL), MX_y1.1 (COL)
- net Col_6: now also MX_6.1 (COL), MX_Macro5.1 (COL), MX_Macro9.1 (COL), MX_c1.1 (COL), MX_f4.1 (COL), MX_k1.1 (COL), MX_left1.1 (COL), MX_pgup1.1 (COL), MX_sclk1.1 (COL), MX_u1.1 (COL)
- net Col_7: now also MX_7.1 (COL), MX_Macro10.1 (COL), MX_Macro3.1 (COL), MX_Macro6.1 (COL), MX_down1.1 (COL), MX_f5.1 (COL), MX_i1.1 (COL), MX_l1.1 (COL), MX_paus1.1 (COL), MX_v1.1 (COL)
- net Col_8: now also MX_8.1 (COL), MX_Macro1.1 (COL), MX_Macro4.1 (COL), MX_b1.1 (COL), MX_caps1.1 (COL), MX_f6.1 (COL), MX_lctl1.1 (COL), MX_o1.1 (COL), MX_rght1.1 (COL), MX_scln1.1 (COL)
- net Col_9: now also MX_9.1 (COL), MX_Macro2.1 (COL), MX_a1.1 (COL), MX_f7.1 (COL), MX_lgui1.1 (COL), MX_n1.1 (COL), MX_p1.1 (COL), MX_quot1.1 (COL), MX_tab1.1 (COL)
- net GND: now also R_0.2, R_1.2, R_2.2, R_3.2, R_4.2, R_5.2, R_6.2, R_7.2, R_8.2, R_9.2, R_Macro1.2, R_Macro10.2, R_Macro2.2, R_Macro3.2, R_Macro4.2, R_Macro5.2, R_Macro6.2, R_Macro7.2, R_Macro8.2, R_Macro9.2, R_a1.2, R_app1.2, R_b1.2, R_bsls1.2, R_bspc1.2, R_c1.2, R_caps1.2, R_comm1.2, R_d1.2, R_del1.2, R_dot1.2, R_down1.2, R_e1.2, R_end1.2, R_ent1.2, R_eql1.2, R_esc1.2, R_f1.2, R_f10.2, R_f11.2, R_f12.2, R_f13.2, R_f2.2, R_f3.2, R_f4.2, R_f5.2, R_f6.2, R_f7.2, R_f8.2, R_f9.2, R_g1.2, R_grv1.2, R_h1.2, R_home1.2, R_i1.2, R_ins1.2, R_j1.2, R_k1.2, R_l1.2, R_lalt1.2, R_lbrc1.2, R_lctl1.2, R_left1.2, R_lgui1.2, R_lsft1.2, R_m1.2, R_mins1.2, R_n1.2, R_o1.2, R_p1.2, R_paus1.2, R_pgdn1.2, R_pgup1.2, R_pscr1.2, R_q1.2, R_quot1.2, R_r1.2, R_ralt1.2, R_rbrc1.2, R_rctl1.2, R_rght1.2, R_rgui1.2, R_rsft1.2, R_s1.2, R_sclk1.2, R_scln1.2, R_slsh1.2, R_spc1.2, R_t1.2, R_tab1.2, R_u1.2, R_up1.2, R_v2.2, R_x1.2, R_y1.2, R_z1.2
- net LED_VIN: now also Q1.2 (D), USB1.11 (VBUS), USB1.2 (VBUS)
- net RO_1_DN: now also U1.2 (GPIO1)
- net Row_0: now also D_esc1.1 (K), D_f1.1 (K), D_f2.1 (K), D_f3.1 (K), D_f4.1 (K), D_f5.1 (K), D_f6.1 (K), D_f7.1 (K), D_re1.1 (K), D_re2.1 (K); no longer SW_re1.S2, SW_re2.S2
- net Row_1: now also D_Macro1.1 (K), D_Macro2.1 (K), D_f10.1 (K), D_f11.1 (K), D_f12.1 (K), D_f8.1 (K), D_f9.1 (K), D_paus1.1 (K), D_pscr1.1 (K), D_sclk1.1 (K)
- net Row_2: now also D_1.1 (K), D_2.1 (K), D_3.1 (K), D_4.1 (K), D_5.1 (K), D_6.1 (K), D_7.1 (K), D_8.1 (K), D_9.1 (K), D_grv1.1 (K)
- net Row_3: now also D_0.1 (K), D_Macro3.1 (K), D_Macro4.1 (K), D_bspc1.1 (K), D_eql1.1 (K), D_home1.1 (K), D_ins1.1 (K), D_mins1.1 (K), D_pgup1.1 (K), D_tab1.1 (K)
- net Row_4: now also D_e1.1 (K), D_i1.1 (K), D_o1.1 (K), D_p1.1 (K), D_q1.1 (K), D_r1.1 (K), D_t1.1 (K), D_u1.1 (K), D_w1.1 (K), D_y1.1 (K)
- net Row_5: now also D_Macro5.1 (K), D_Macro6.1 (K), D_a1.1 (K), D_bsls1.1 (K), D_caps1.1 (K), D_del1.1 (K), D_end1.1 (K), D_lbrc1.1 (K), D_pgdn1.1 (K), D_rbrc1.1 (K)
- net Row_6: now also D_d1.1 (K), D_f13.1 (K), D_g1.1 (K), D_h1.1 (K), D_j1.1 (K), D_k1.1 (K), D_l1.1 (K), D_quot1.1 (K), D_s1.1 (K), D_scln1.1 (K)
- net Row_7: now also D_Macro7.1 (K), D_Macro8.1 (K), D_b1.1 (K), D_c1.1 (K), D_ent1.1 (K), D_lsft1.1 (K), D_n1.1 (K), D_v1.1 (K), D_x1.1 (K), D_z1.1 (K)
- net Row_8: now also D_Macro10.1 (K), D_Macro9.1 (K), D_comm1.1 (K), D_dot1.1 (K), D_lctl1.1 (K), D_lgui1.1 (K), D_m1.1 (K), D_rsft1.1 (K), D_slsh1.1 (K), D_up1.1 (K)
- net Row_9: now also D_app1.1 (K), D_down1.1 (K), D_lalt1.1 (K), D_left1.1 (K), D_ralt1.1 (K), D_rctl1.1 (K), D_rght1.1 (K), D_rgui1.1 (K), D_spc1.1 (K)
- net V_USB_IN: no longer Q1.2 (D), USB1.11 (VBUS), USB1.2 (VBUS)
- removed net LED_VOUT: R_0.2, R_1.2, R_2.2, R_3.2, R_4.2, R_5.2, R_6.2, R_7.2, R_8.2, R_9.2, R_Macro1.2, R_Macro10.2, R_Macro2.2, R_Macro3.2, R_Macro4.2, R_Macro5.2, R_Macro6.2, R_Macro7.2, R_Macro8.2, R_Macro9.2, R_a1.2, R_app1.2, R_b1.2, R_bsls1.2, R_bspc1.2, R_c1.2, R_caps1.2, R_comm1.2, R_d1.2, R_del1.2, R_dot1.2, R_down1.2, R_e1.2, R_end1.2, R_ent1.2, R_eql1.2, R_esc1.2, R_f1.2, R_f10.2, R_f11.2, R_f12.2, R_f13.2, R_f2.2, R_f3.2, R_f4.2, R_f5.2, R_f6.2, R_f7.2, R_f8.2, R_f9.2, R_g1.2, R_grv1.2, R_h1.2, R_home1.2, R_i1.2, R_ins1.2, R_j1.2, R_k1.2, R_l1.2, R_lalt1.2, R_lbrc1.2, R_lctl1.2, R_left1.2, R_lgui1.2, R_lsft1.2, R_m1.2, R_mins1.2, R_n1.2, R_o1.2, R_p1.2, R_paus1.2, R_pgdn1.2, R_pgup1.2, R_pscr1.2, R_q1.2, R_quot1.2, R_r1.2, R_ralt1.2, R_rbrc1.2, R_rctl1.2, R_rght1.2, R_rgui1.2, R_rsft1.2, R_s1.2, R_sclk1.2, R_scln1.2, R_slsh1.2, R_spc1.2, R_t1.2, R_tab1.2, R_u1.2, R_up1.2, R_v2.2, R_w1.2, R_x1.2, R_y1.2, R_z1.2
- new net: D_re1.2 (A), SW_re1.S2
- new net: D_re2.2 (A), SW_re2.S2
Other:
- moved on the sheet: D_0, D_1, D_2, D_3, D_4, D_5, D_6, D_7, D_8, D_9, D_Macro1, D_Macro10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
